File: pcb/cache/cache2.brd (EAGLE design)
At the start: 87.6 x 86 mm, 9 parts

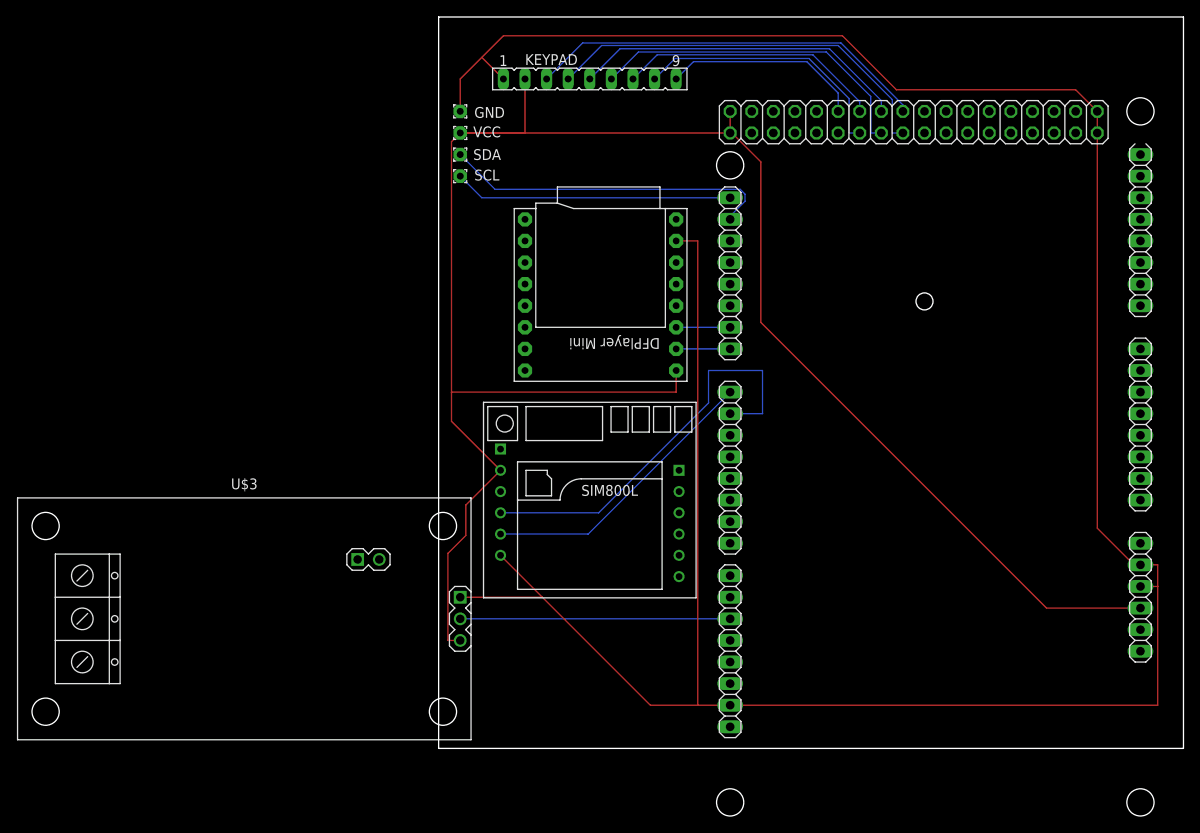
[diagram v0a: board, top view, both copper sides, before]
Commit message: updated pcb
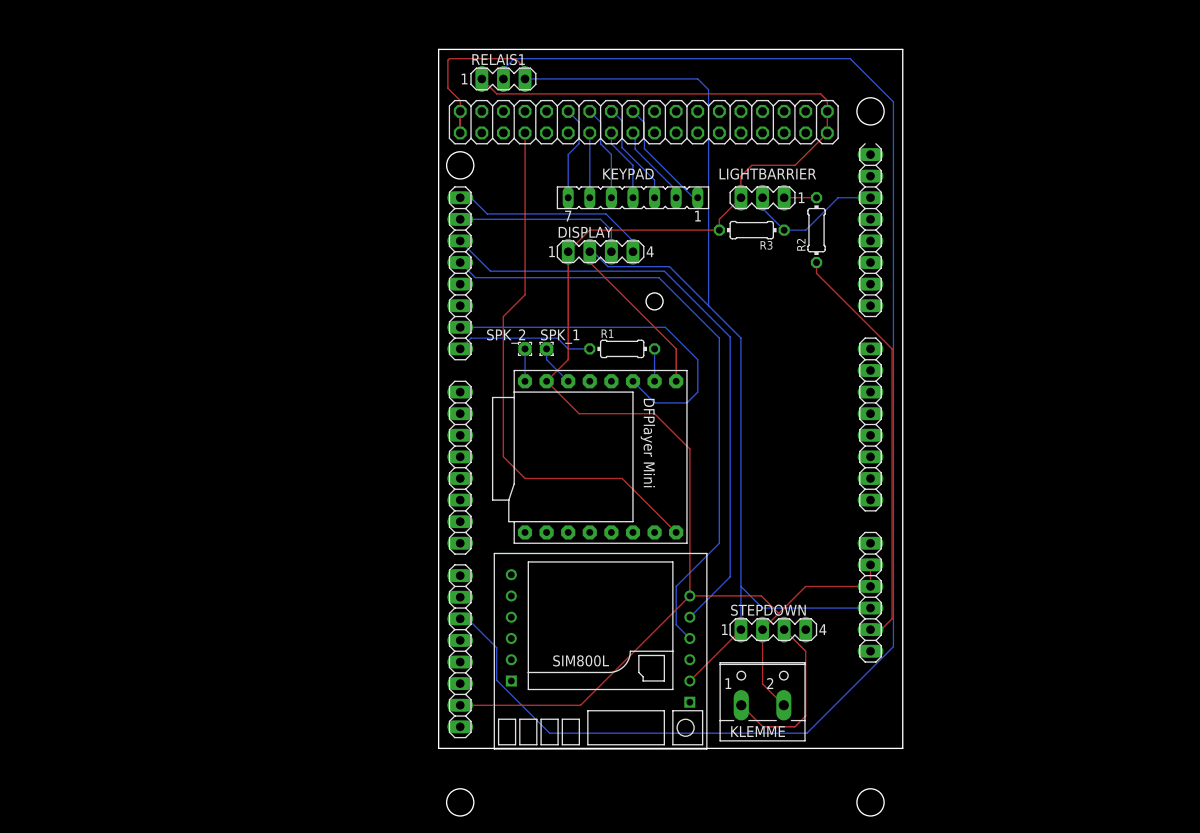
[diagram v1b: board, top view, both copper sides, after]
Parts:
- removed GND, SCL, SDA, VCC: (no value), wirepad:1,6/0,8
- removed U$3: RELAY-1-SRD, diy-modules:RELAY-1-SRD
- added DISPLAY, STEPDOWN: (no value), con-lstb:MA04-1
- added KLEMME: (no value), con-wago-500:W237-102
- added LIGHTBARRIER, RELAIS1: (no value), con-lstb:MA03-1
- added R1, R2, R3: (no value), rcl:0204/7
- added SPK_1, SPK_2: (no value), wirepad:1,6/0,8
- KEYPAD: device con-lsta:FE09 -> con-lsta:FE07
- moved IC1 31.8 mm to (53.3, -21.6)
- moved U$1 19.1 mm to (19.1, 34.3), turned to 270 degrees
- moved U$2 17.8 mm to (19.1, 11.4), turned to 180 degrees
- moved KEYPAD 14.9 mm to (22.9, 64.8), turned to 180 degrees
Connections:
- removed net +3V3: IC1.2
- removed net VCC.2: U$3.J2.2
- new net 3V3: LIGHTBARRIER.1, R2.2
- new net IN+: KLEMME.1, STEPDOWN.3
- new net IN-B: IC1.20, LIGHTBARRIER.2, R3.1
- new net N$15: R1.2, U$1.RX
- new net N$16: IC1.2, R2.1
- new net N$17: SPK_2.1, U$1.SPK2
- new net N$18: SPK_1.1, U$1.SPK1
- new net N$19: IC1.53, U$1.BUSY
- net +5V: now also DISPLAY.2, RELAIS1.3, STEPDOWN.1; no longer KEYPAD.2, U$3.J1.3, VCC.1
- net GND: now also DISPLAY.1, KLEMME.2, LIGHTBARRIER.3, R3.2, RELAIS1.1, STEPDOWN.2; no longer GND.1, KEYPAD.1, U$3.J1.1
- net N$1: now also IC1.25; no longer IC1.31
- net N$10: now also KEYPAD.3; no longer KEYPAD.5
- net N$11: now also KEYPAD.2; no longer KEYPAD.4
- net N$12: now also KEYPAD.1; no longer KEYPAD.3
- net N$13: now also R1.1; no longer U$1.RX
- net N$2: now also IC1.26; no longer IC1.32
- net N$3: now also RELAIS1.2; no longer U$3.J1.2
- net N$4: now also DISPLAY.3; no longer SDA.1
- net N$5: now also DISPLAY.4; no longer SCL.1
- net N$6: now also KEYPAD.7; no longer KEYPAD.9
- net N$7: now also KEYPAD.6; no longer KEYPAD.8
- net N$8: now also KEYPAD.5; no longer KEYPAD.7
- net N$9: now also KEYPAD.4; no longer KEYPAD.6
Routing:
- net N$3: track 31.8 -> 176.7 mm
- net GND: track 316.0 -> 208.6 mm
- net N$19: track 0.00 -> 63.2 mm
- net +5V: track 226.5 -> 171.9 mm
- net N$16: track 0.00 -> 48.7 mm
- net N$11: track 47.6 -> 9.72 mm
- net N$1: track 33.9 -> 71.4 mm
- net N$14: track 6.35 -> 42.5 mm
- net N$12: track 47.4 -> 13.6 mm
- net N$9: track 39.5 -> 8.67 mm
- net N$10: track 39.6 -> 12.3 mm
- net N$7: track 31.1 -> 7.62 mm
- net N$2: track 48.9 -> 72.3 mm
- net IN+: track 0.00 -> 20.4 mm
- net N$8: track 31.3 -> 11.2 mm
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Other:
- board size 87.6 x 86 mm -> 54.6 x 82.2 mm
